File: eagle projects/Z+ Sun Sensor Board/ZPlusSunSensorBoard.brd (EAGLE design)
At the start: 78 x 78 mm, 54 parts, among them J1 Power In, J2 Power Out, U1 TSV991AILT, U2 ADS7841E_2K5, U4 LM20BIM7X_NOPB, U5 TSV991AILT, U8 TSV991AILT

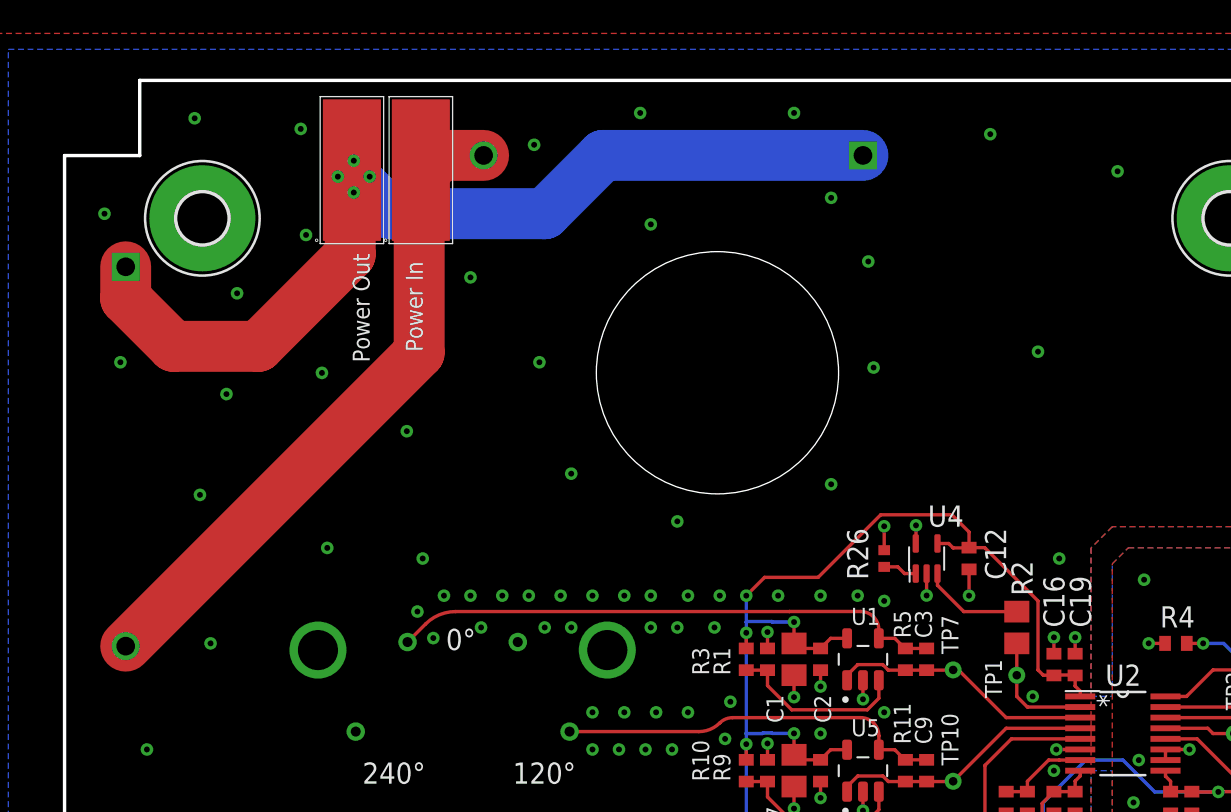
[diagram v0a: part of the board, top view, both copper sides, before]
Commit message: dumb dumb fix dumb mistake
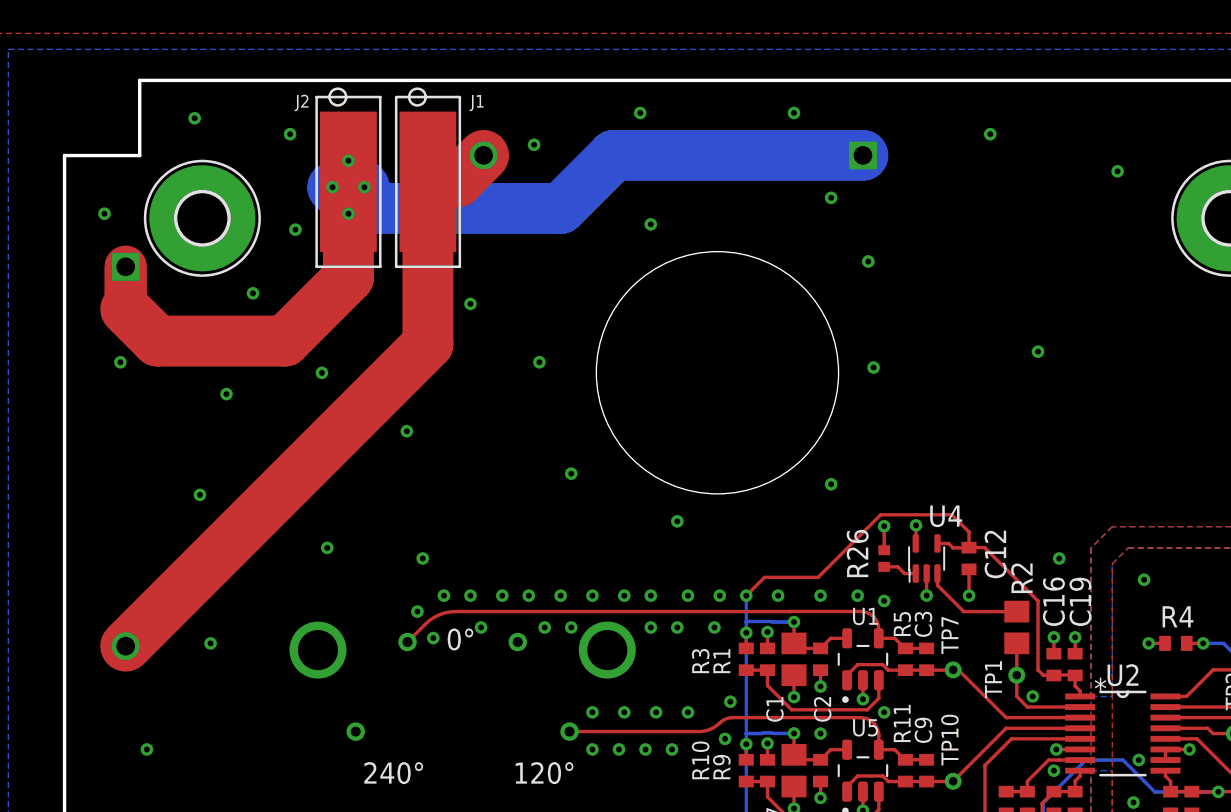
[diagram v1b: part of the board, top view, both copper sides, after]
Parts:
- moved J2 8.24 mm to (21.6, 82.2), turned to 270 degrees
- moved J1 7.96 mm to (26.4, 82.2), turned to 270 degrees
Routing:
- net N$6: track 62.1 -> 61.1 mm
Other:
- board text removed: "Power In"
- board text removed: "Power Out"
